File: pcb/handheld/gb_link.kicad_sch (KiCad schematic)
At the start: 25 parts, among them J6 Link_Port, U18 74LVC1T45

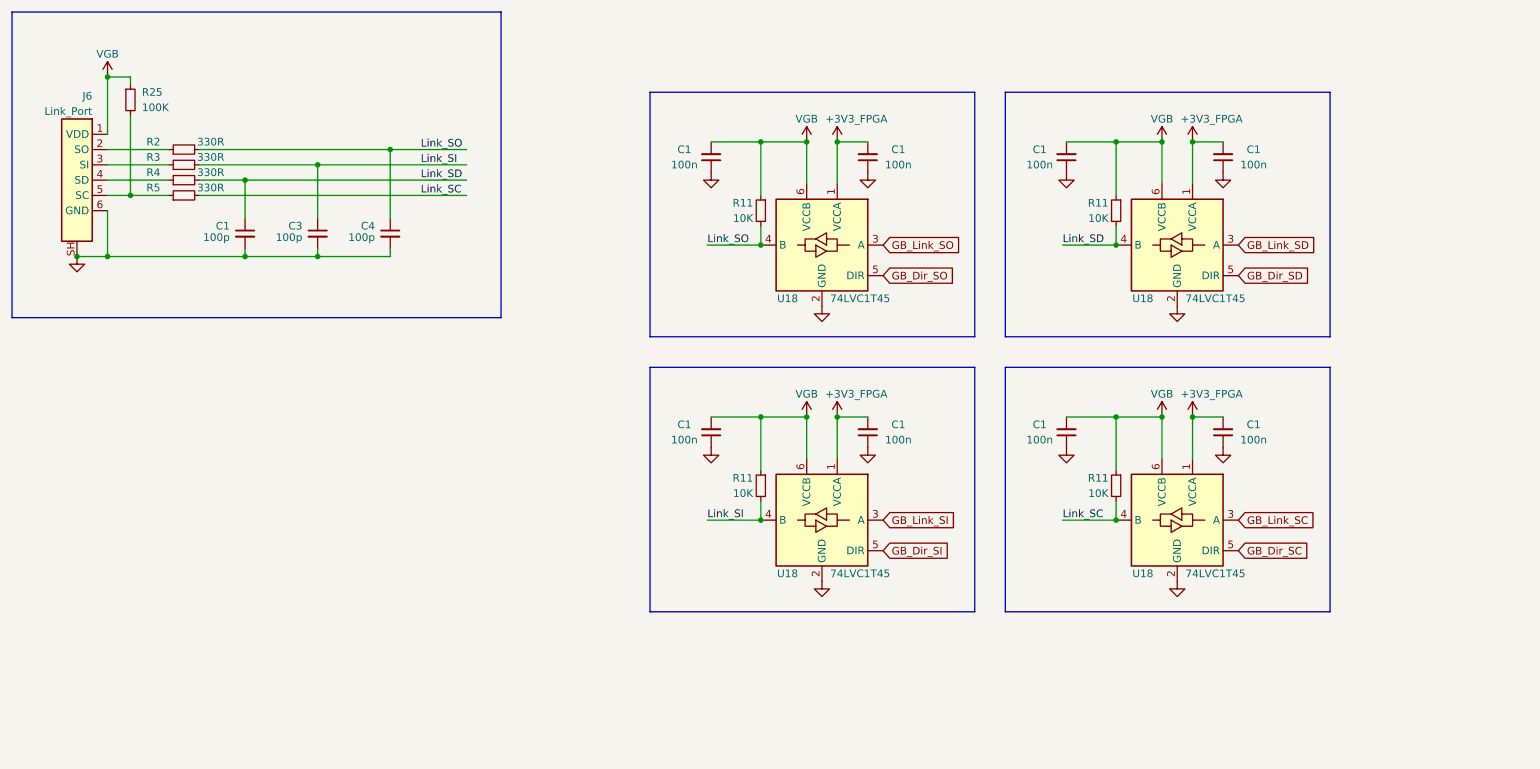
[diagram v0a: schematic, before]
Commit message: Rev A of PCB
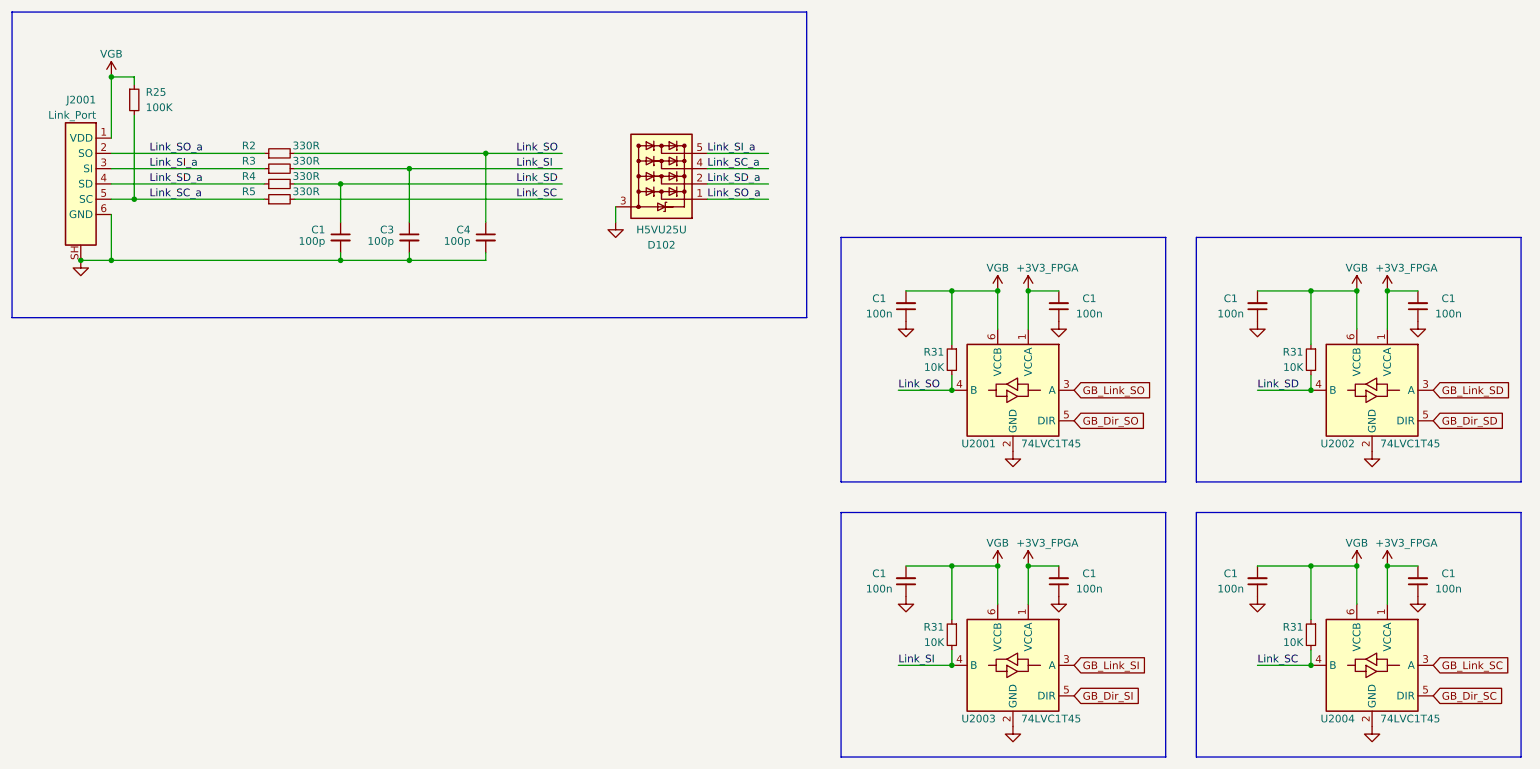
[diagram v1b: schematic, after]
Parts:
- added D102: H5VU25U, Package_DFN_QFN:Diodes_UDFN-10_1.0x2.5mm_P0.5mm, symbol Game_Bub:H5VU25U
- J2001: renamed from J6; footprint (none) -> Game_Bub:GameBoy_LinkPort_AGB_Horizontal
- U2001, U2002, U2003, U2004: renamed from U18; LCSC C168855 -> C5162250
- renumbered R11 to R31
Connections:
- net GND: now also D102.3 (A), D102.8 (A)
- net Link_SD_a: now reaches J2001.4 (SD), R4.1
- net Link_SD_a: now also D102.2 (K2), D102.9 (K2)
- net Link_SO_a: now reaches J2001.2 (SO), R2.1
- net Link_SO_a: now also D102.1 (K1), D102.10 (K1)
- net Link_SI_a: now reaches J2001.3 (SI), R3.1
- net Link_SI_a: now also D102.5 (K4), D102.6 (K4)
- net Link_SC_a: now reaches J2001.5 (SC), R25.2, R5.1
- net Link_SC_a: now also D102.4 (K3), D102.7 (K3)
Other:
- moved on the sheet: C1, C3, C4, J2001, R2, R25, R3, R31, R4, R5, U2001, U2002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
